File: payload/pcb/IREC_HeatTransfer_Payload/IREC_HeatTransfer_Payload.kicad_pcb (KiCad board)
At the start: 2 copper layers, 63.5 x 104.1 mm, 41 parts, among them J1 XT60PW-M, J2 Screw_Terminal_01x02, J3 Screw_Terminal_01x02, J4 Screw_Terminal_01x02, J5 Screw_Terminal_01x02, U1 MAX31855KASA, U2 DS18B20, U3 DEV-16771, U4 MAX31855KASA, U5 MAX31855KASA, U7 AP63357

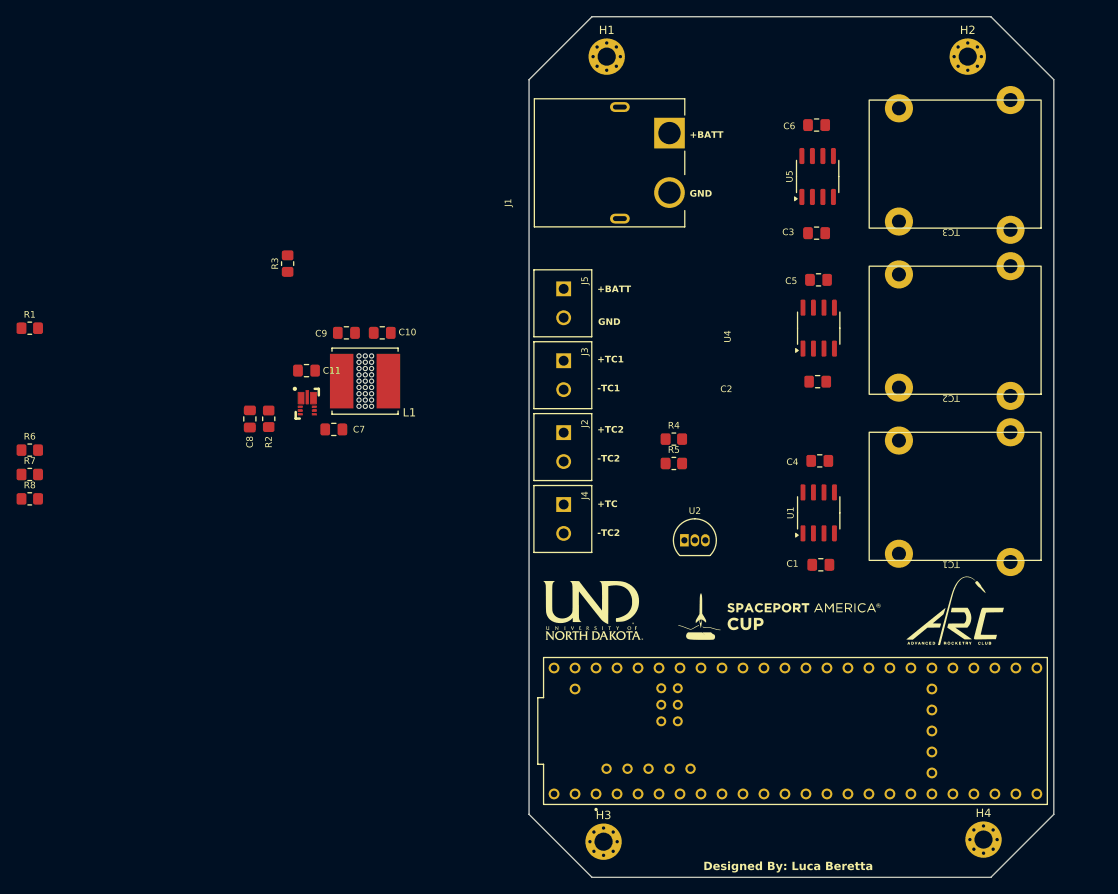
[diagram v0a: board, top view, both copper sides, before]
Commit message: updates to pcb
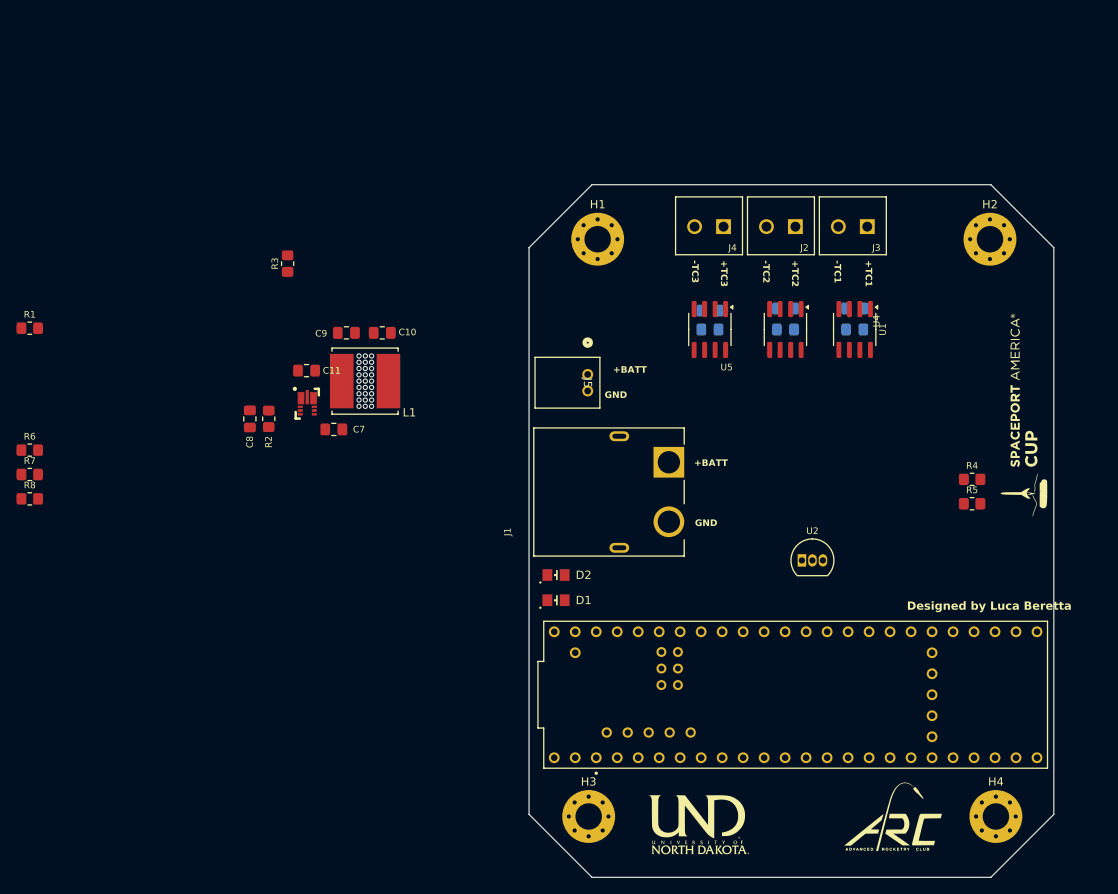
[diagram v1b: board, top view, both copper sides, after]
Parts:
- removed TC1, TC2, TC3: Thermocouple_Block, CustomFootprintLib:PCC-SMP-K
- added D1: OSRAM_LGR971-KN-1, Skyhawkson_Footprints:OSRAM_0805, F.Cu at (163.3, 101.1)
- added D2: OSRAM_LSR976-NR-1, Skyhawkson_Footprints:OSRAM_0805, F.Cu at (163.3, 98.0)
- C1, C2, C3, C4, C5, C6: moved to B.Cu
- H1, H2, H3, H4: footprint MountingHole:MountingHole_2.2mm_M2_Pad_Via -> MountingHole:MountingHole_3.2mm_M3_Pad_Via
- J5: value Screw_Terminal_01x02 -> S2B-PH-K-SLFSN; footprint CustomFootprintLib:TERMBLOCK_OSTTE020104_3_5MM -> CustomFootprintLib:CONN_S2B-PH-K-S_JST
- moved J1 39.8 mm to (170.9, 88.0)
- moved J4 39.5 mm to (181.8, 55.9), turned to 180 degrees
- moved J3 39.3 mm to (199.2, 55.9), turned to 180 degrees
- moved G*** 38.4 mm to (220.0, 78.7), turned to 90 degrees
- moved J2 37.5 mm to (190.5, 55.9), turned to 180 degrees
- moved R4 36.4 mm to (213.6, 86.5)
- moved R5 36.4 mm to (213.6, 89.4)
- moved C1 31.3 mm to (199.4, 65.8), turned to 0 degrees
- moved G*** 28.9 mm to (180.6, 128.3)
- moved C6 27.9 mm to (181.9, 68.3), turned to 0 degrees
- moved G*** 26.0 mm to (204.0, 127.8)
- moved U5 22.6 mm to (181.9, 68.3), turned to -90 degrees
- moved U1 22.6 mm to (199.4, 68.3), turned to -90 degrees
- moved H2 22.3 mm to (215.8, 57.4)
- moved H1 22.1 mm to (168.3, 57.4)
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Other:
- board size 63.5 x 104.1 mm -> 63.5 x 83.8 mm
- board text added: "+TC3"
- board text added: "-TC3"
- board text added: "Designed by Luca Beretta"
- board text removed: "+TC"
- board text removed: "Designed By: Luca Beretta"
